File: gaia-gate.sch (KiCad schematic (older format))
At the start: 38 parts, among them J1 motor, J2 230V_IN, J3 Home_Controller, J4 Open_Close_Sensor, J5 Extras, K1 SANYOU_SRD_Form_C, K2 SANYOU_SRD_Form_C, Q1 BC547, Q2 BC547, U1 Vcc_one_supply, U2 ATmega328P-PU, U3 Current_Transformer, U4 LM741, Y1 Crystal

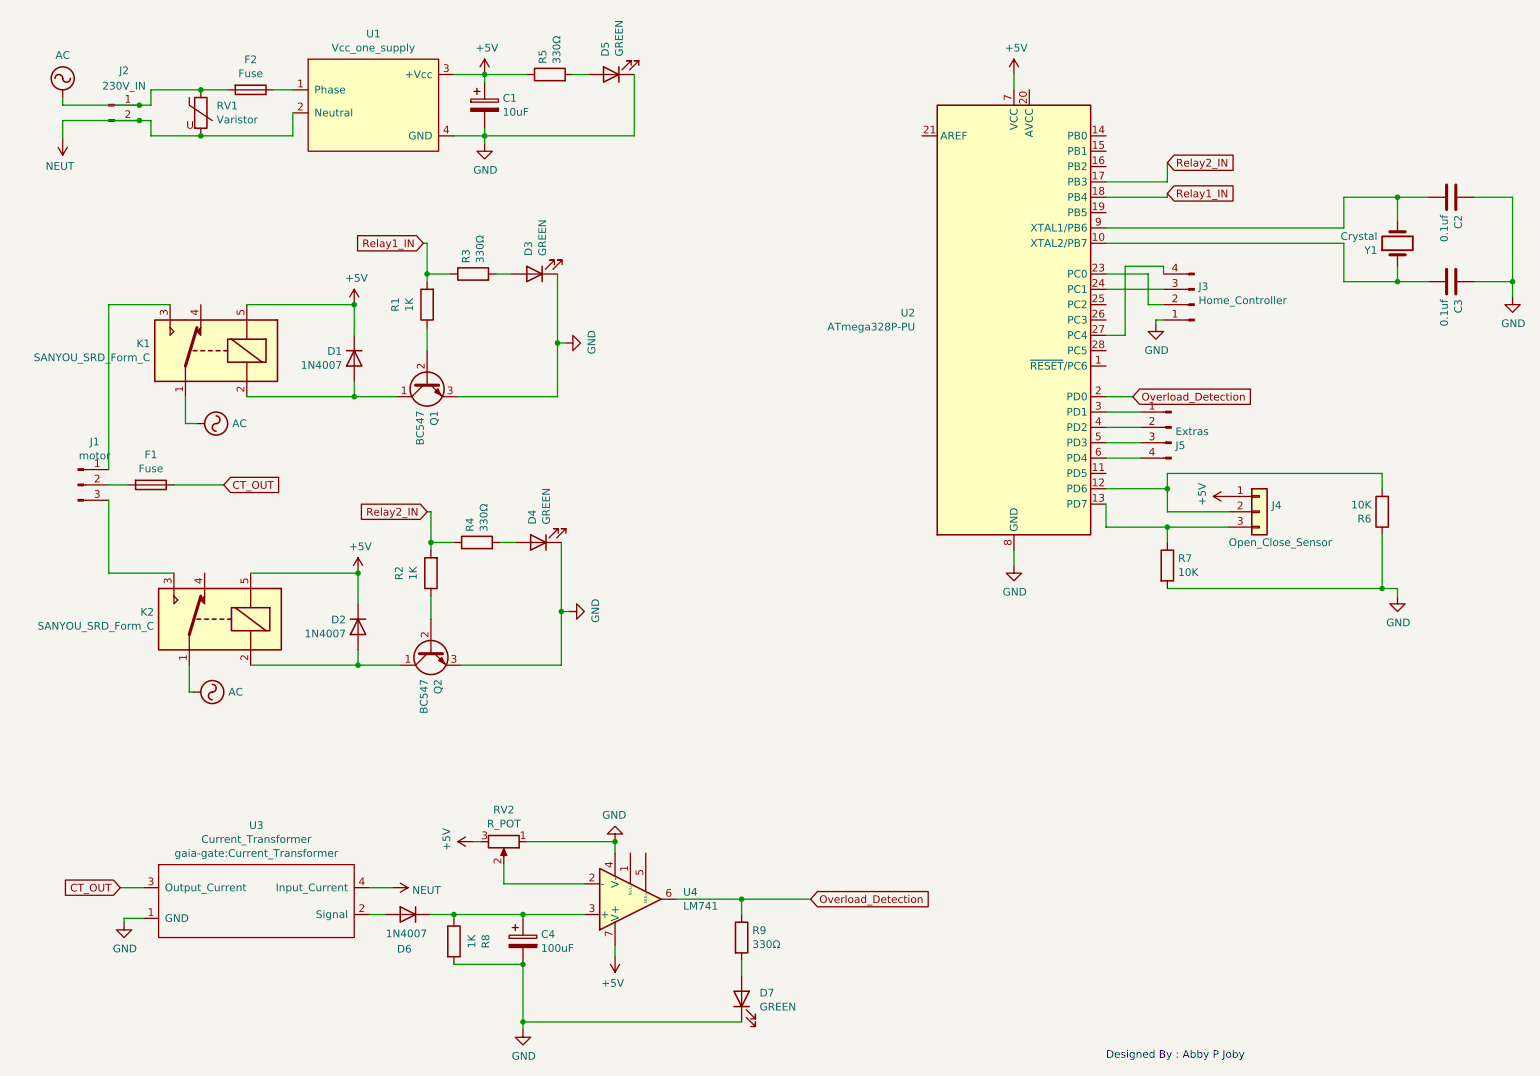
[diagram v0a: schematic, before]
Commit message: latest pcb
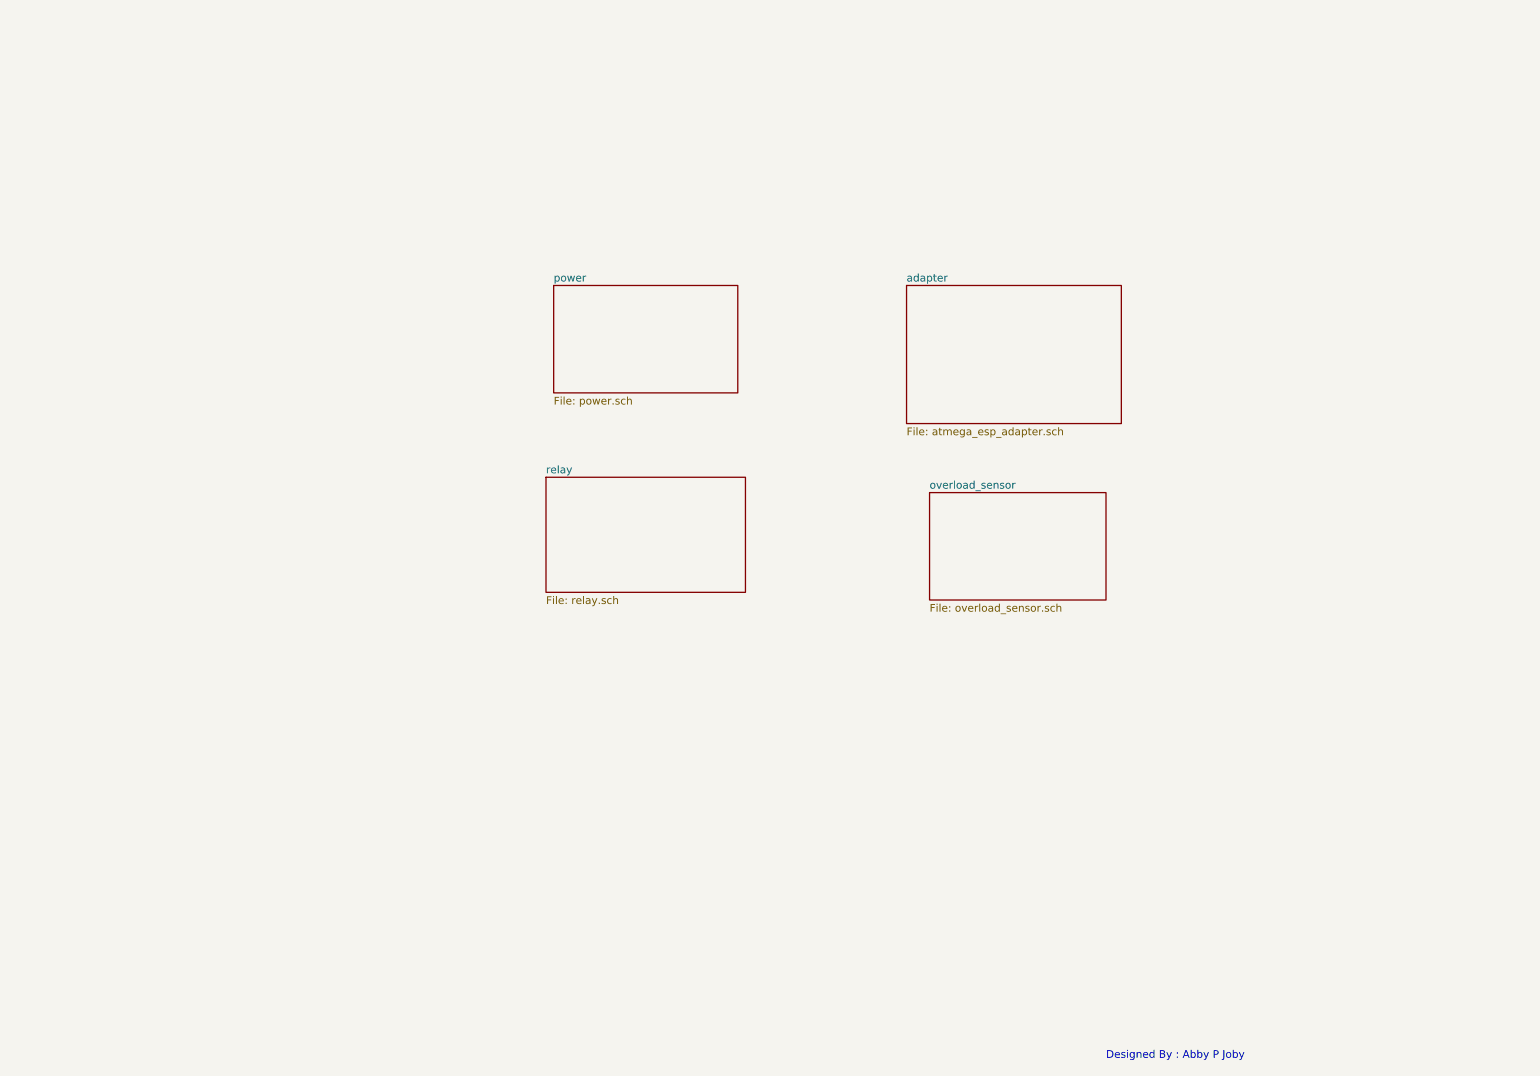
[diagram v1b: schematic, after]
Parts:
- removed C1: 10uF, Capacitor_THT:CP_Radial_D8.0mm_P5.00mm, symbol Device:CP
- removed C2, C3: 0.1uf, Capacitor_THT:C_Disc_D3.8mm_W2.6mm_P2.50mm, symbol Device:C
- removed C4: 100uF, Capacitor_THT:CP_Radial_D8.0mm_P5.00mm, symbol Device:CP
- removed D1, D2, D6: 1N4007, Diode_THT:D_DO-41_SOD81_P10.16mm_Horizontal, symbol Diode:1N4007
- removed D3, D4, D5, D7: GREEN, LED_THT:LED_D5.0mm, symbol Device:LED
- removed F1, F2: Fuse, gaia-gate:Fuse, symbol Device:Fuse
- removed J1: motor, Connector_Molex:Molex_KK-396_A-41791-0003_1x03_P3.96mm_Vertical, symbol Connector:Conn_01x03_Male
- removed J2: 230V_IN, Connector_Molex:Molex_KK-396_A-41791-0002_1x02_P3.96mm_Vertical, symbol Connector:Conn_01x02_Male
- removed J3: Home_Controller, Connector_Molex:Molex_KK-254_AE-6410-04A_1x04_P2.54mm_Vertical, symbol Connector:Conn_01x04_Male
- removed J4: Open_Close_Sensor, Connector_Molex:Molex_KK-254_AE-6410-03A_1x03_P2.54mm_Vertical, symbol Connector_Generic:Conn_01x03
- removed J5: Extras, Connector_Molex:Molex_KK-254_AE-6410-04A_1x04_P2.54mm_Vertical, symbol Connector:Conn_01x04_Male
- removed K1, K2: SANYOU_SRD_Form_C, Relay_THT:Relay_SPDT_SANYOU_SRD_Series_Form_C, symbol Relay:SANYOU_SRD_Form_C
- removed Q1, Q2: BC547, Package_TO_SOT_THT:TO-92_Inline_Wide, symbol Transistor_BJT:BC547
- removed R1, R2, R8: 1K, gaia-gate:resistor, symbol Device:R
- removed R3, R4, R5, R9: 330Ω, gaia-gate:resistor, symbol Device:R
- removed R6, R7: 10K, gaia-gate:resistor, symbol Device:R
- removed RV1: Varistor, Varistor:RV_Disc_D9mm_W6.1mm_P5mm, symbol Device:Varistor
- removed RV2: R_POT, Potentiometer_THT:Potentiometer_Bourns_3296W_Vertical, symbol Device:R_POT
- removed U1: Vcc_one_supply, gaia-gate:230_5V_supply_HiLink, symbol pcb_power_supply:Vcc_one_supply
- removed U2: ATmega328P-PU, Package_DIP:DIP-28_W7.62mm_Socket_LongPads, symbol MCU_Microchip_ATmega:ATmega328P-PU
- removed U3: Current_Transformer, gaia-gate:Current_Transformer, symbol gaia_library:Current_Transformer
- removed U4: LM741, Package_DIP:DIP-8_W10.16mm_LongPads, symbol Amplifier_Operational:LM741
- removed Y1: Crystal, Crystal:Crystal_HC18-U_Vertical, symbol Device:Crystal
